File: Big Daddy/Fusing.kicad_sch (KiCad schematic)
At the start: 24 parts, among them K1 T9VV1K15-12S, Q3 IXFH34N65X2, Q4 IXFH34N65X2, U11 LM5050-1, U12 LM5050-1, U4 LT1528CQ#PBF

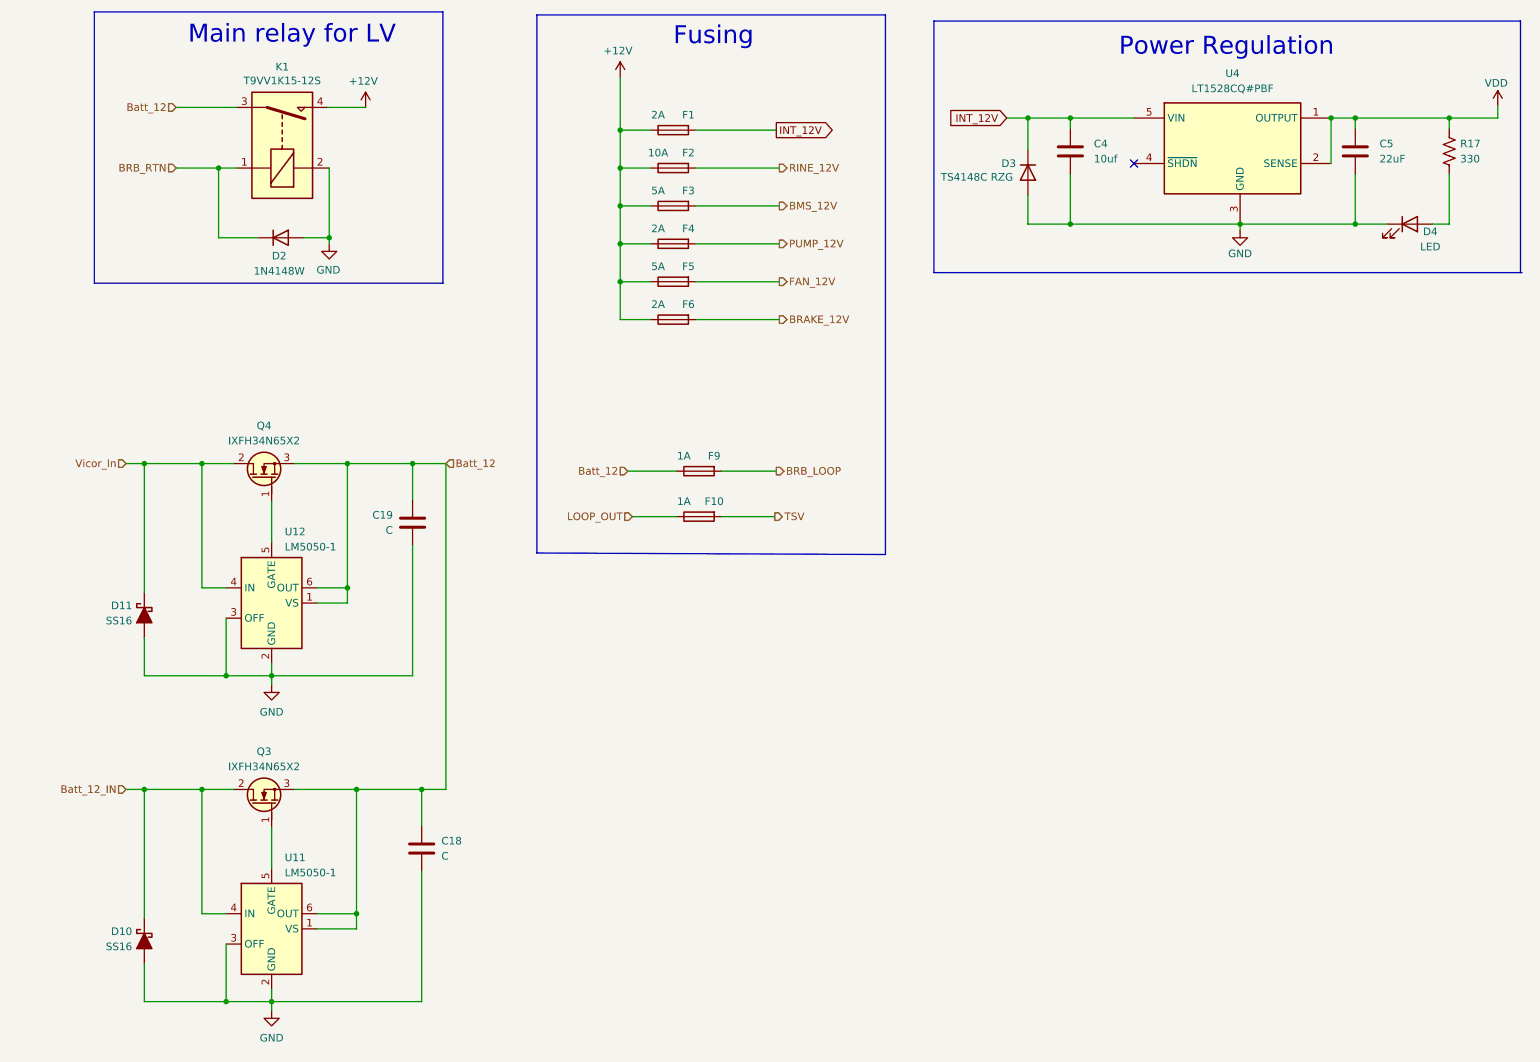
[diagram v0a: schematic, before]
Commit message: Schematic DONE
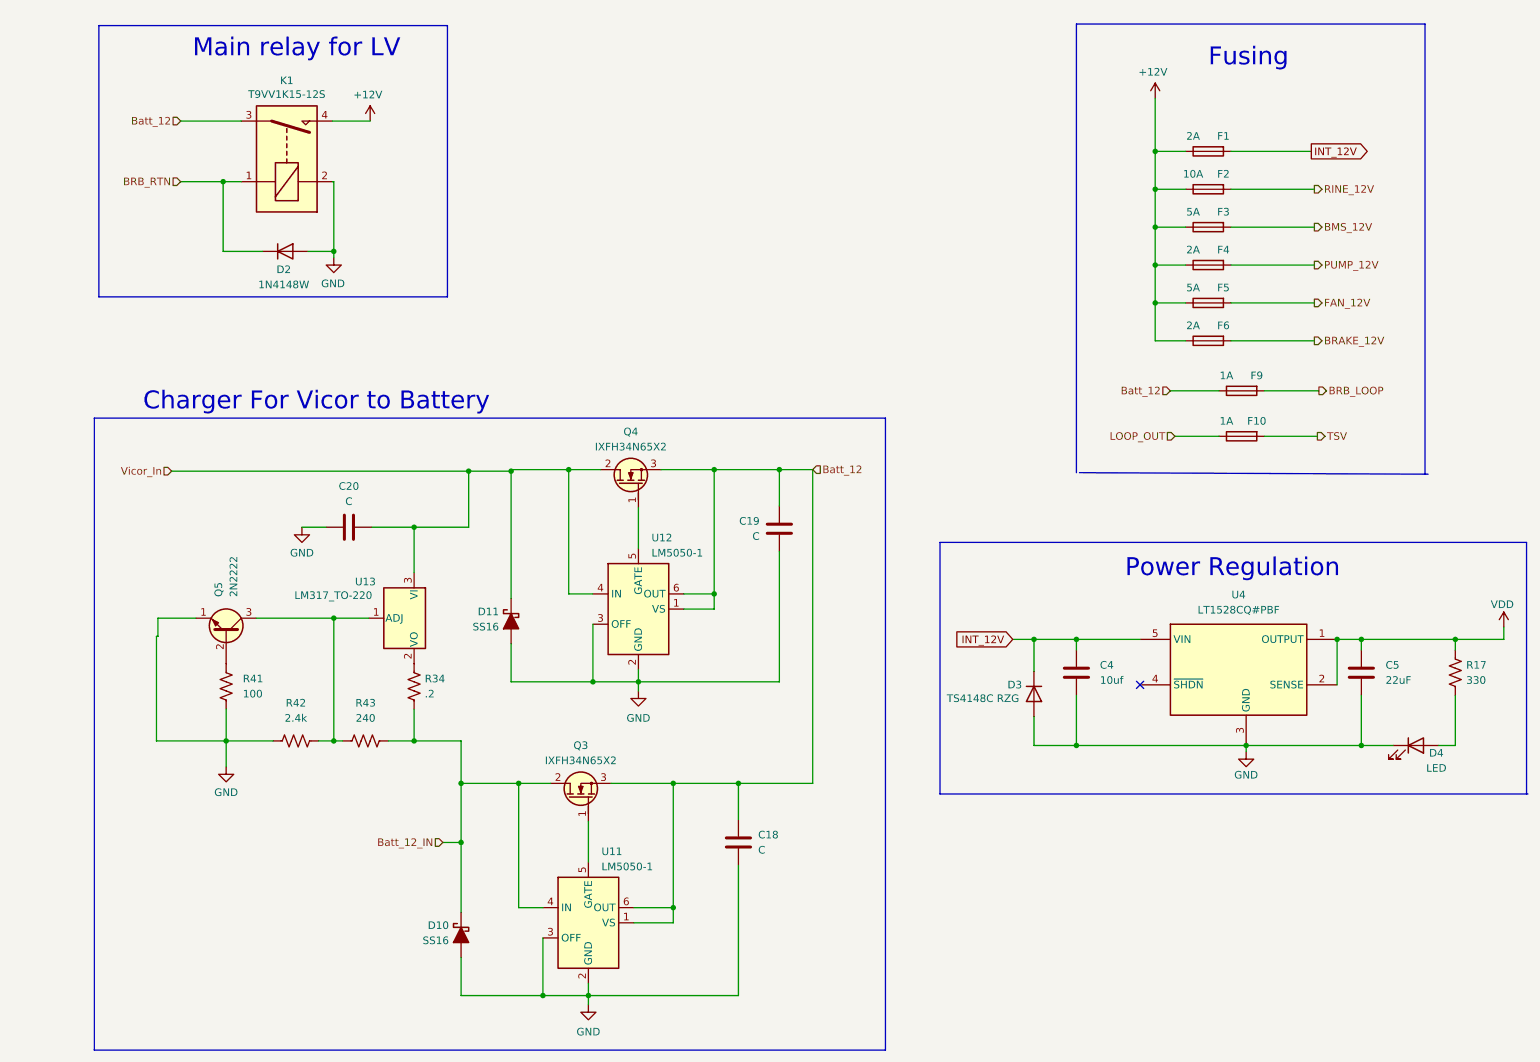
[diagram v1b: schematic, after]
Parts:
- added C20: C, symbol Device:C
- added Q5: 2N2222, Package_TO_SOT_THT_AKL:TO-18-3_EBC, symbol PCM_Transistor_BJT_AKL:2N2222
- added R34: .2, symbol Device:R_US
- added R41: 100, symbol Device:R_US
- added R42: 2.4k, symbol Device:R_US
- added R43: 240, symbol Device:R_US
- added U13: LM317_TO-220, Package_TO_SOT_THT:TO-220-3_Vertical, symbol Regulator_Linear:LM317_TO-220
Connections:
- net Batt_12_IN: now also R34.1, R43.2
- net GND: now also C20.2, Q5.1 (E), R41.2, R42.1
- net Vicor_In: now also C20.1, U13.3 (VI)
- new net: Q5.3 (C), R42.2, R43.1, U13.1 (ADJ)
- new net: R34.2, U13.2 (VO)
- new net: Q5.2 (B), R41.1
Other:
- note added: "Charger For Vicor to Battery"
- moved on the sheet: C18, C19, C4, C5, D10, D11, D2, D3, D4, F1, F10, F2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
